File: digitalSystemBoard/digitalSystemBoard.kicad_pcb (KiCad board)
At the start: 2 copper layers, 194 parts, among them J1 Barrel_Jack, J10 Conn_02x03_Odd_Even, J11 Conn_02x03_Odd_Even, J12 Conn_02x03_Odd_Even, J2 USB-B, J3 Conn_02x04_Odd_Even, J4 Conn_02x04_Odd_Even, J5 Conn_02x08_Odd_Even, J6 Conn_02x07_Odd_Even, J7 Conn_02x07_Odd_Even, J8 Conn_02x08_Odd_Even, J9 Conn_02x03_Odd_Even, Q1 MJD122T4G, Q10 BC847, Q11 BC847, Q12 BC847, Q13 BC847, Q14 BC847, Q15 BC847, Q16 BC847, Q17 BC847, Q2 BC847, Q3 BC847, Q4 BC847, Q5 BC847, Q6 BC847, Q7 BC847, Q8 BC847, Q9 BC847, SW1 SW_SPDT, SW9 ButtonFirst, U1 LM317, U10 IO_Switch, U11 IO_Switch, U12 IO_Switch, U13 IO_Switch, U14 74LS04, U15 Potentiometer, U16 ATmega32U4-AU, U17 ICSP, U18 74LS165, U19 74HC164, U2 KCSA02-105, U20 74LS165, U21 74HC164, U3 KCSA02-105, U4 74LS47, U5 74LS47, U6 IO_Switch, U7 IO_Switch, U8 IO_Switch, U9 IO_Switch, Y1 16MHz

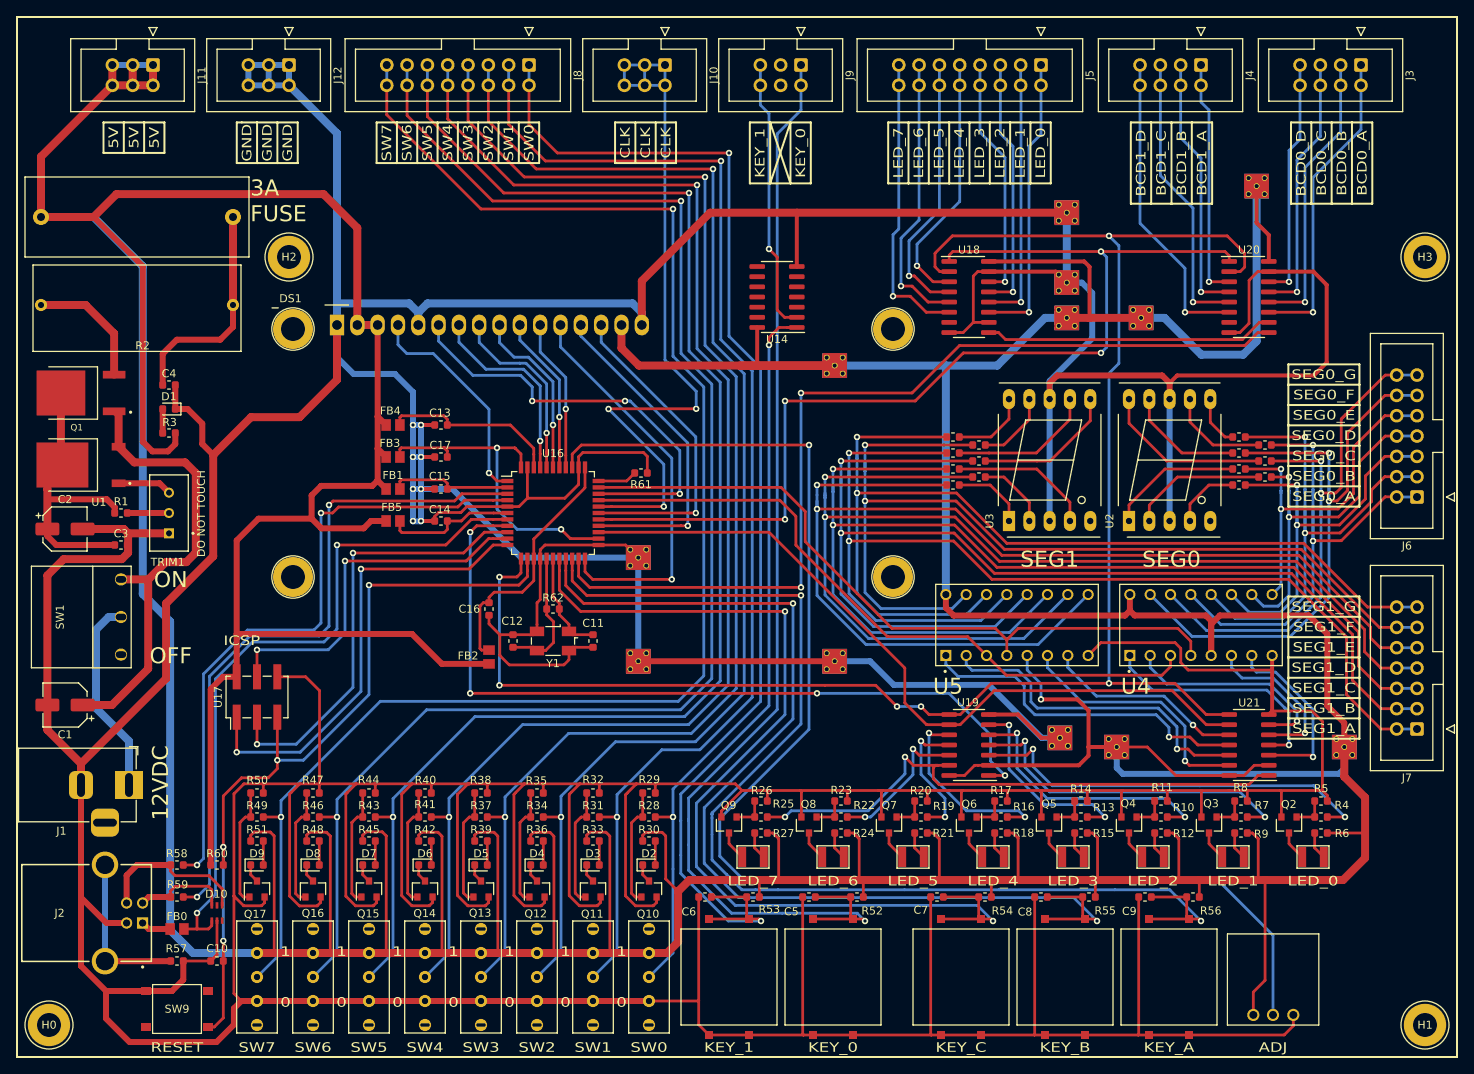
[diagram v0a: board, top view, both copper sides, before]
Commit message: re-route power line, reset origin
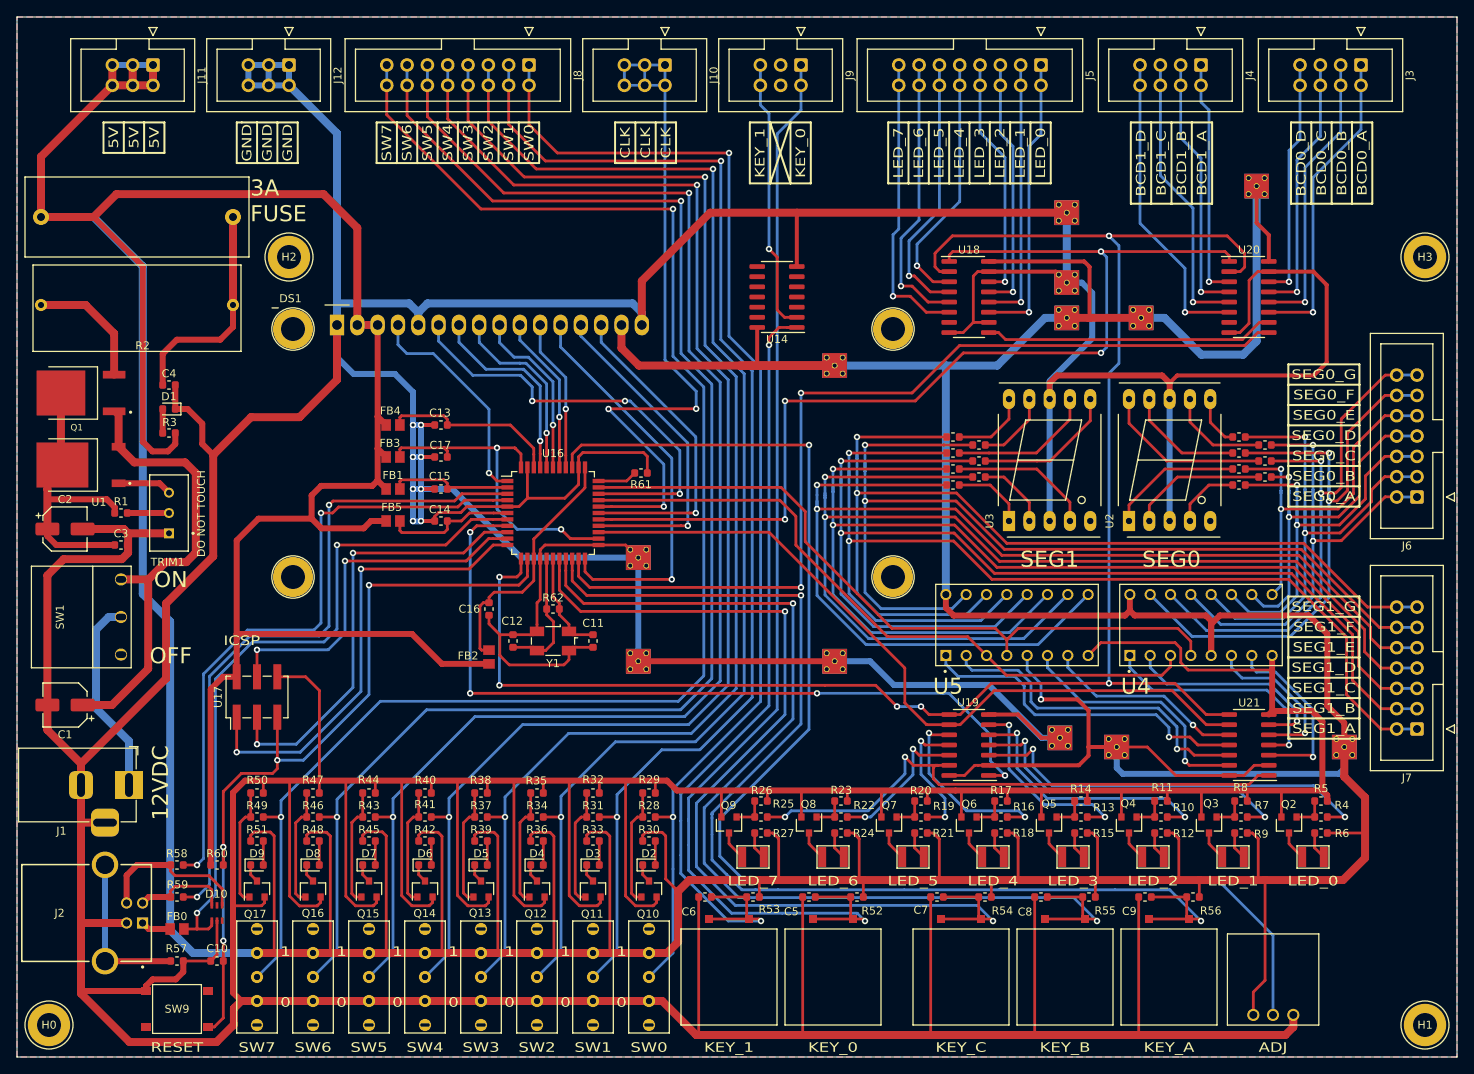
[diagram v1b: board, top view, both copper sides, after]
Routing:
- net GND: track 1457.9 -> 1464.6 mm
- added copper zone on B.Cu, net GND
- added copper zone on F.Cu, net GND
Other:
- board outline added: 180 x 130 mm
